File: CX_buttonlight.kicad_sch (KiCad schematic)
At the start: 10 parts, among them U1 LM317L_SOT-89

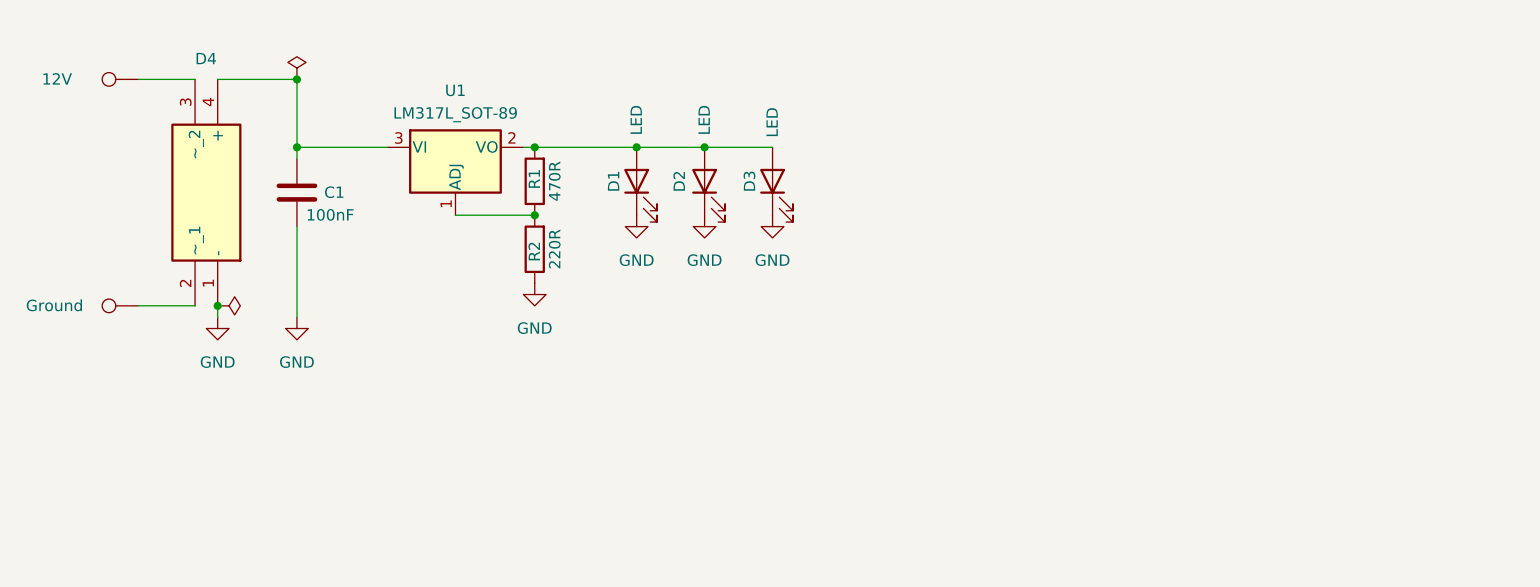
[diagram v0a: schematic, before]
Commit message: Tweaks og tekster
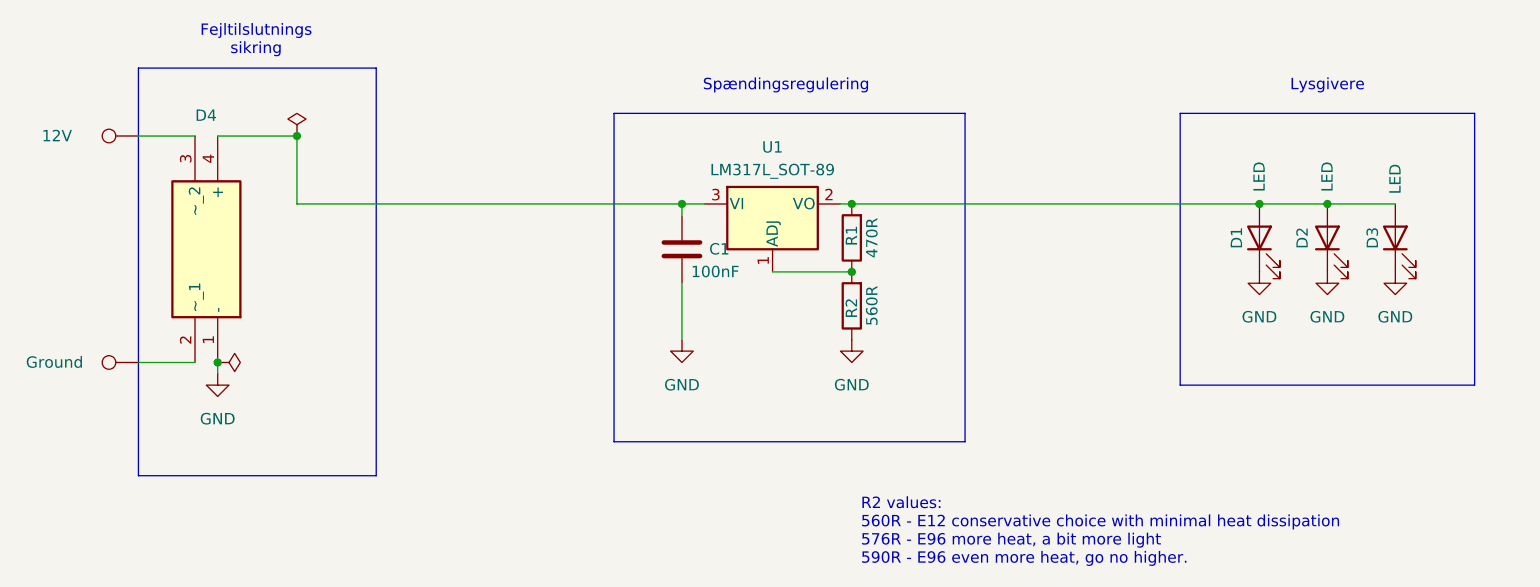
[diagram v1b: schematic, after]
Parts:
- R2: value 220R -> 560R
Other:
- note added: "Fejltilslutnings sikring"
- note added: "Lysgivere"
- note added: "R2 values: 560R - E12 conservative choice with minimal heat dissipation 576R - E96 more heat, a bit more light 590R - E96 even more heat, go no higher."
- note added: "Spændingsregulering"
- company: (none) -> PowerStation
- title: (none) -> CX vippeknap-lys
- moved on the sheet: C1, D1, D2, D3, D4, R1, R2, U1
